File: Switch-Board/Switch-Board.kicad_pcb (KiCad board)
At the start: 2 copper layers, 75.5 x 71 mm, 20 parts, among them J1 Conn_01x08_Pin, J2 Conn_01x08_Pin, J3 Conn_01x08_Pin, J4 Conn_01x08_Pin, SW1 SW_Nidec_CAS-120A1, SW10 SW_Nidec_CAS-120A1, SW11 SW_Nidec_CAS-120A1, SW12 SW_Nidec_CAS-120A1, SW13 SW_Nidec_CAS-120A1, SW14 SW_Nidec_CAS-120A1, SW15 SW_Nidec_CAS-120A1, SW16 SW_Nidec_CAS-120A1, SW2 SW_Nidec_CAS-120A1, SW3 SW_Nidec_CAS-120A1, SW4 SW_Nidec_CAS-120A1, SW5 SW_Nidec_CAS-120A1, SW6 SW_Nidec_CAS-120A1, SW7 SW_Nidec_CAS-120A1, SW8 SW_Nidec_CAS-120A1, SW9 SW_Nidec_CAS-120A1

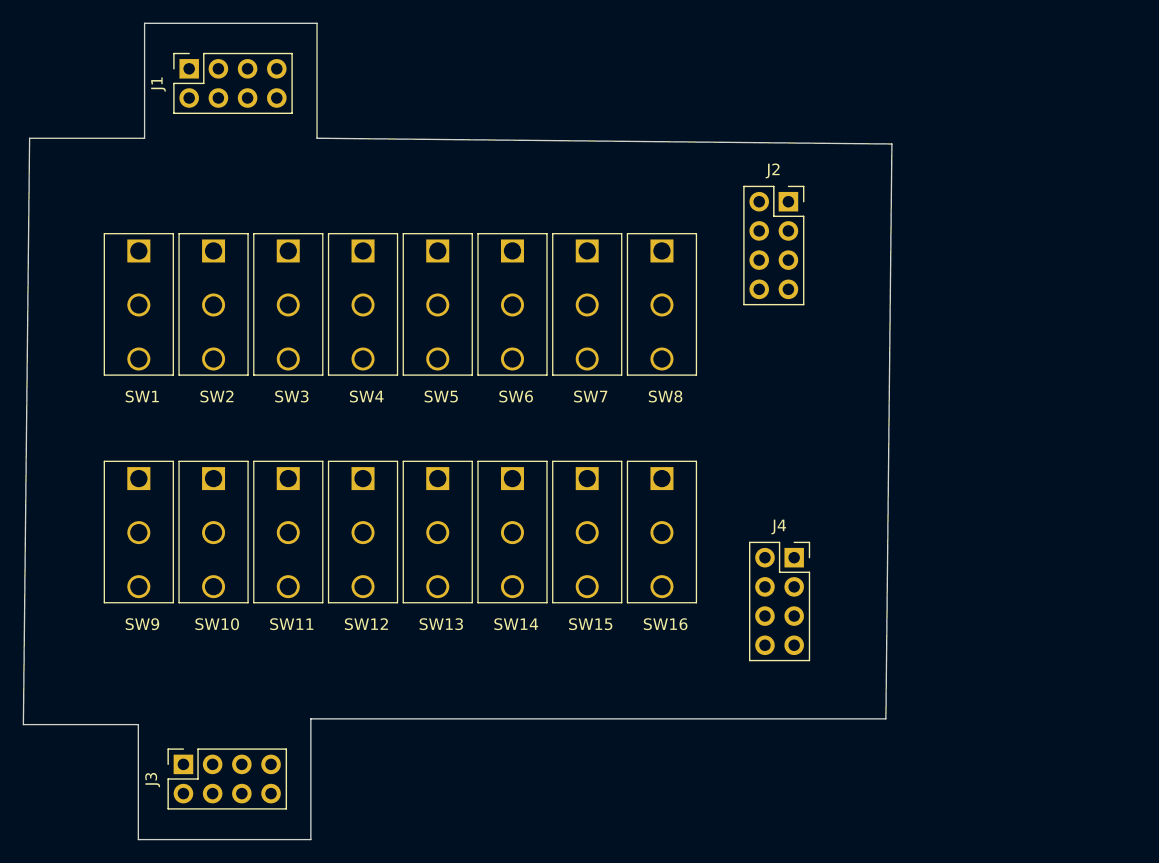
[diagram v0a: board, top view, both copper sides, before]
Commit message: Finished Switch Board
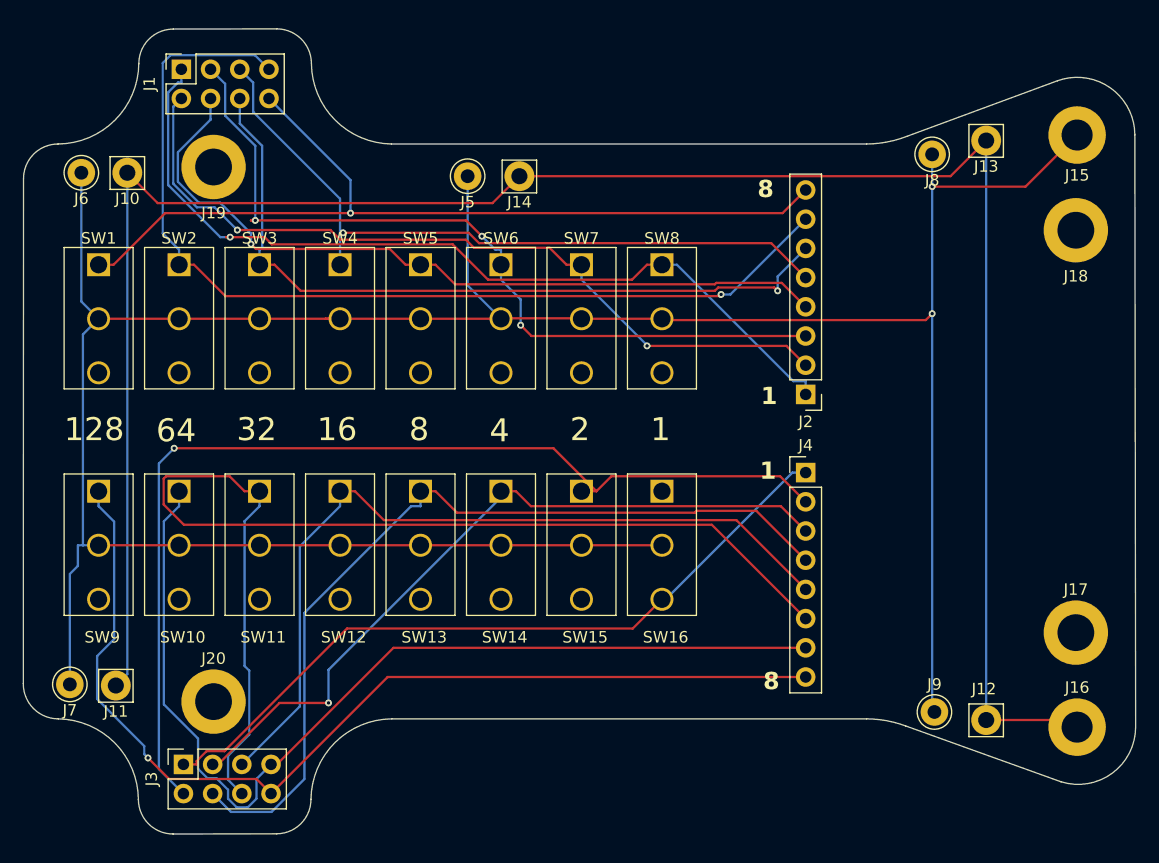
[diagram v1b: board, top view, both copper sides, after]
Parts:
- added J10: Conn_01x01_Pin, Connector_Pin:Pin_D1.4mm_L8.5mm_W2.8mm_FlatFork, F.Cu at (43.5, 32.5)
- added J11: Conn_01x01_Pin, Connector_Pin:Pin_D1.4mm_L8.5mm_W2.8mm_FlatFork, F.Cu at (42.5, 77.1)
- added J12: Conn_01x01_Pin, Connector_Pin:Pin_D1.4mm_L8.5mm_W2.8mm_FlatFork, F.Cu at (118.2, 80.1)
- added J13: Conn_01x01_Pin, Connector_Pin:Pin_D1.4mm_L8.5mm_W2.8mm_FlatFork, F.Cu at (118.2, 29.7)
- added J14: Conn_01x01_Pin, Connector_Pin:Pin_D1.4mm_L8.5mm_W2.8mm_FlatFork, F.Cu at (77.6, 32.8)
- added J15: Conn_01x01_Pin, MountingHole:MountingHole_2.5mm_Pad, F.Cu at (126.1, 29.2)
- added J16: Conn_01x01_Pin, MountingHole:MountingHole_2.5mm_Pad, F.Cu at (126.1, 80.7)
- added J17: Conn_01x01_Pin, MountingHole:MountingHole_3.2mm_M3_DIN965_Pad, F.Cu at (126.0, 72.5)
- added J18: Conn_01x01_Pin, MountingHole:MountingHole_3.2mm_M3_DIN965_Pad, F.Cu at (126.0, 37.5)
- added J19: Conn_01x01_Pin, MountingHole:MountingHole_3.2mm_M3_DIN965_Pad, F.Cu at (51.0, 32.0)
- added J20: Conn_01x01_Pin, MountingHole:MountingHole_3.2mm_M3_DIN965_Pad, F.Cu at (51.0, 78.5)
- added J5: Conn_01x01_Pin, Connector_Pin:Pin_D1.0mm_L10.0mm_LooseFit, F.Cu at (73.1, 32.8)
- added J6: Conn_01x01_Pin, Connector_Pin:Pin_D1.0mm_L10.0mm_LooseFit, F.Cu at (39.5, 32.5)
- added J7: Conn_01x01_Pin, Connector_Pin:Pin_D1.0mm_L10.0mm_LooseFit, F.Cu at (38.5, 77.0)
- added J8: Conn_01x01_Pin, Connector_Pin:Pin_D1.0mm_L10.0mm_LooseFit, F.Cu at (113.5, 30.9)
- added J9: Conn_01x01_Pin, Connector_Pin:Pin_D1.0mm_L10.0mm_LooseFit, F.Cu at (113.7, 79.4)
- J2, J4: footprint Connector_PinSocket_2.54mm:PinSocket_2x04_P2.54mm_Vertical -> Connector_PinHeader_2.54mm:PinHeader_1x08_P2.54mm_Vertical
- moved J2 16.8 mm to (102.5, 51.8), turned to 180 degrees
- moved J4 7.47 mm to (102.5, 58.6)
- moved SW1 3.70 mm to (41.0, 45.2)
- moved SW9 3.67 mm to (41.0, 64.9)
- moved SW2 3.23 mm to (48.0, 45.2)
- moved SW10 3.20 mm to (48.0, 64.9)
- moved SW3 2.77 mm to (55.0, 45.2)
- moved SW11 2.73 mm to (55.0, 64.9)
- moved SW4 2.33 mm to (62.0, 45.2)
- moved SW12 2.28 mm to (62.0, 64.9)
- moved SW5 1.92 mm to (69.0, 45.2)
- moved SW13 1.86 mm to (69.0, 64.9)
- moved SW6 1.56 mm to (76.0, 45.2)
- moved SW14 1.49 mm to (76.0, 64.9)
- moved SW7 1.30 mm to (83.0, 45.2)
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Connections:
- SW1 pad 1: Net-(J1-Pin_1) -> Net-(J1-Pin_8)
- SW10 pad 1: Net-(J3-Pin_2) -> Net-(J3-Pin_7)
- SW11 pad 1: Net-(J3-Pin_3) -> Net-(J3-Pin_6)
- SW12 pad 1: Net-(J3-Pin_4) -> Net-(J3-Pin_5)
- SW13 pad 1: Net-(J3-Pin_5) -> Net-(J3-Pin_4)
- SW14 pad 1: Net-(J3-Pin_6) -> Net-(J3-Pin_3)
- SW15 pad 1: Net-(J3-Pin_7) -> Net-(J3-Pin_2)
- SW16 pad 3: Net-(J3-Pin_8) -> Net-(J3-Pin_1)
- SW2 pad 1: Net-(J1-Pin_2) -> Net-(J1-Pin_7)
- SW3 pad 1: Net-(J1-Pin_3) -> Net-(J1-Pin_6)
- SW4 pad 1: Net-(J1-Pin_4) -> Net-(J1-Pin_5)
- SW5 pad 1: Net-(J1-Pin_5) -> Net-(J1-Pin_4)
- SW6 pad 1: Net-(J1-Pin_6) -> Net-(J1-Pin_3)
- SW7 pad 1: Net-(J1-Pin_7) -> Net-(J1-Pin_2)
- SW8 pad 1: Net-(J1-Pin_8) -> Net-(J1-Pin_1)
- SW9 pad 1: Net-(J3-Pin_1) -> Net-(J3-Pin_8)
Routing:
- net +5V: track 0.00 -> 247.5 mm, vias 0 -> 2
- net GND: track 0.00 -> 181.6 mm
- net Net-(J3-Pin_6): track 0.00 -> 99.4 mm
- net Net-(J3-Pin_2): track 0.00 -> 90.7 mm, vias 0 -> 1
- net Net-(J3-Pin_8): track 0.00 -> 88.9 mm, vias 0 -> 1
- net Net-(J1-Pin_7): track 0.00 -> 87.4 mm, vias 0 -> 1
- net Net-(J3-Pin_7): track 0.00 -> 87.4 mm
- net Net-(J1-Pin_8): track 0.00 -> 77.1 mm, vias 0 -> 1
- net Net-(J1-Pin_1): track 0.00 -> 76.1 mm, vias 0 -> 1
- net Net-(J3-Pin_4): track 0.00 -> 75.9 mm
- net Net-(J3-Pin_5): track 0.00 -> 71.3 mm
- net Net-(J1-Pin_3): track 0.00 -> 71.1 mm, vias 0 -> 3
- net Net-(J1-Pin_2): track 0.00 -> 70.2 mm, vias 0 -> 2
- net Net-(J1-Pin_4): track 0.00 -> 68.2 mm, vias 0 -> 1
- net Net-(J1-Pin_6): track 0.00 -> 66.7 mm, vias 0 -> 1
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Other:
- board size 75.5 x 71 mm -> 96.7 x 70 mm
- board text added: "1"
- board text added: "128"
- board text added: "16"
- board text added: "2"
- board text added: "32"
- board text added: "4"
- board text added: "64"
- board text added: "8"
